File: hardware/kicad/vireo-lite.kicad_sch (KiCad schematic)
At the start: 0 parts

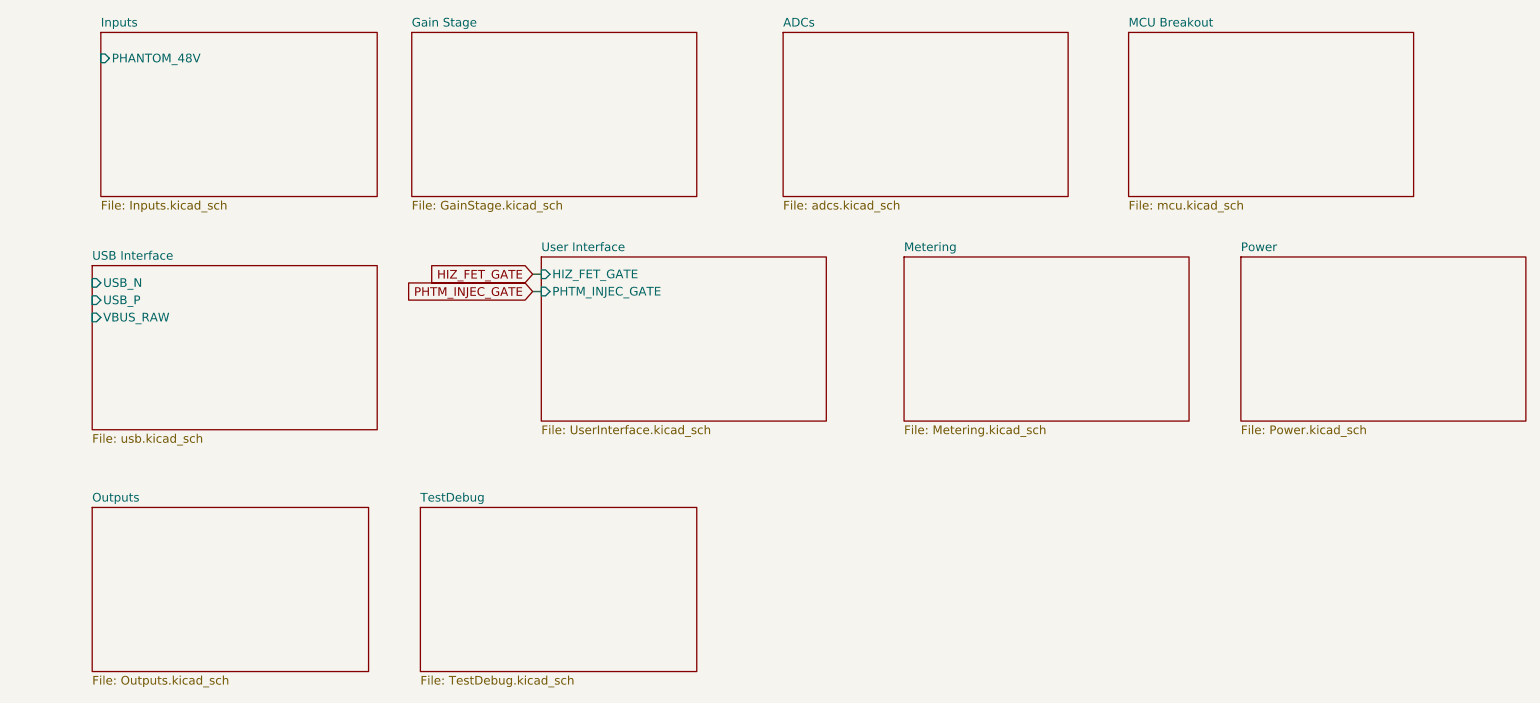
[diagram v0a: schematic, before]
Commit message: stm32h723 breakout
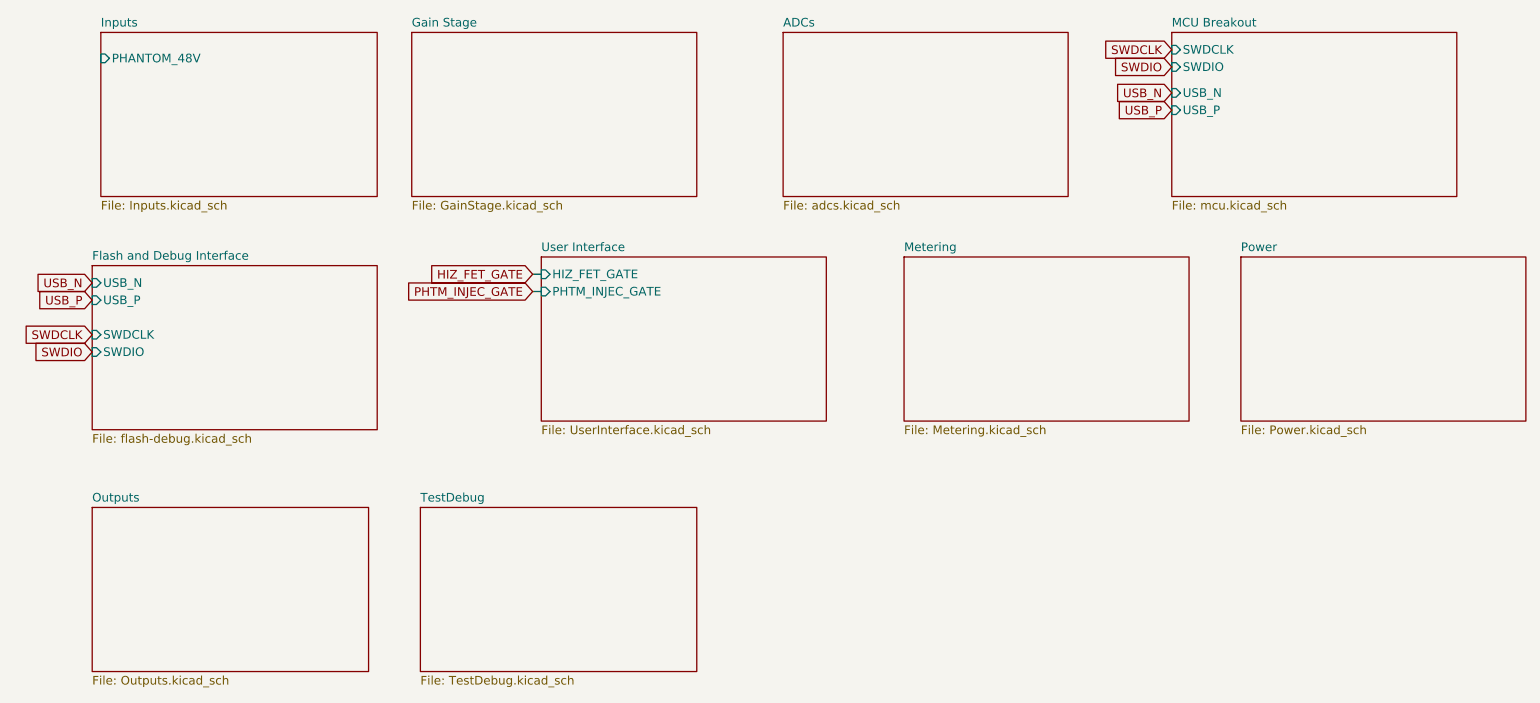
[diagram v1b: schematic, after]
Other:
- sheet USB Interface renamed Flash and Debug Interface
- sheet Flash and Debug Interface: file usb.kicad_sch -> flash-debug.kicad_sch
- sheet Flash and Debug Interface ports: added SWDCLK, SWDIO; removed VBUS_RAW
- sheet MCU Breakout ports: added SWDCLK, SWDIO, USB_N, USB_P; removed none
